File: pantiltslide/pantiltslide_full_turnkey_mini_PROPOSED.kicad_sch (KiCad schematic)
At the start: 64 parts, among them J1 Conn_01x22_Socket, J17 Motor_Slide, J18 Motor_Pan, J19 Motor_Tilt, J2 Conn_01x22_Socket, J20 TCA9548A_Mux, J21 AS5600_Pan, J22 AS5600_Tilt, J23 OLED, J24 TCA9548A_Mux, J26 Limit_Min, J27 Limit_Max, J28 Motor_Aux, J29 Enc_Slide, J3 MUX_2, J30 Enc_Pan, J31 Enc_Tilt, J32 Enc_Aux, J33 Btn_SetKeyframe, J34 Btn_ClearKeyframe, J35 Btn_PlayPause, J36 Btn_Reset, J37 5V_In, J38 24V_In, J4 MUX_3, J41 Aux_Max, J5 MUX_4, J6 MUX_5, J7 MUX_6, J8 MUX_7, U1 tmc2209, U2 tmc2209, U3 tmc2209, U4 tmc2209

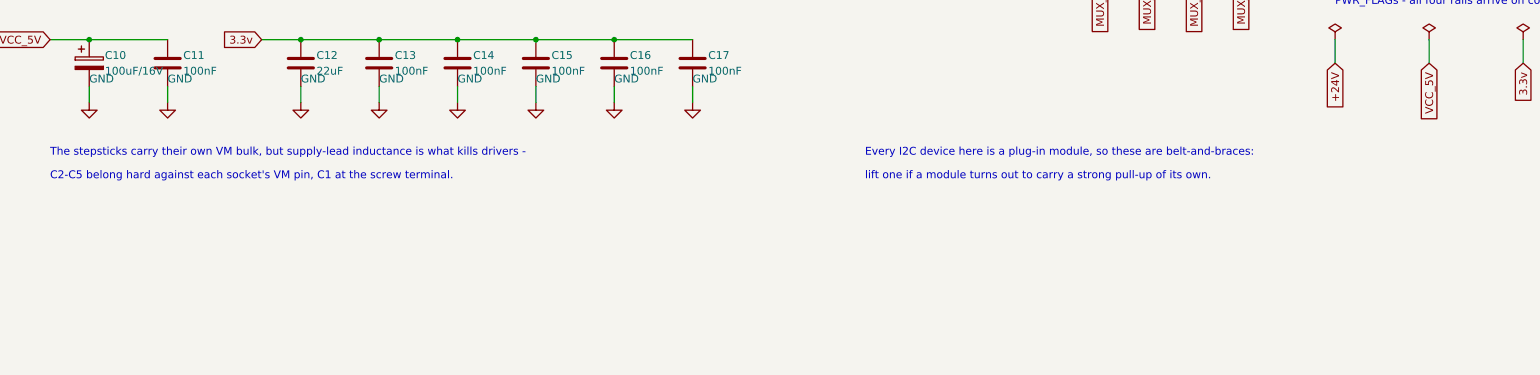
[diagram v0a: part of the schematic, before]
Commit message: new version of board with more caps and res
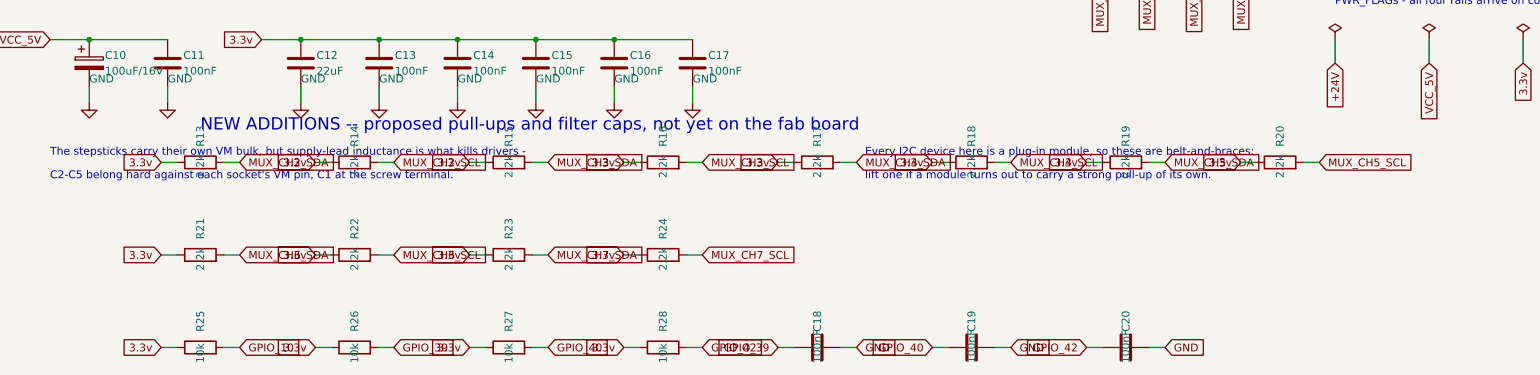
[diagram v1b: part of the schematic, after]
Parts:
- added C18, C19, C20: 100nF, Capacitor_SMD:C_0805_2012Metric, symbol Device:C
- added R13, R14, R15, R16, R17, R18, R19, R20, R21, R22, R23, R24: 2.2k, Resistor_SMD:R_0805_2012Metric, symbol Device:R
- added R25, R26, R27, R28: 10k, Resistor_SMD:R_0805_2012Metric, symbol Device:R
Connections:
- net +3.3V: now also R13.1, R14.1, R15.1, R16.1, R17.1, R18.1, R19.1, R20.1, R21.1, R22.1, R23.1, R24.1, R25.1, R26.1, R27.1, R28.1
- net GND: now also C18.2, C19.2, C20.2
- net GPIO_10: now also R25.2
- net GPIO_39: now also C18.1, R26.2
- net GPIO_40: now also C19.1, R27.2
- net GPIO_42: now also C20.1, R28.2
- net MUX_CH2_SCL: now also R14.2
- net MUX_CH2_SDA: now also R13.2
- net MUX_CH3_SCL: now also R16.2
- net MUX_CH3_SDA: now also R15.2
- net MUX_CH4_SCL: now also R18.2
- net MUX_CH4_SDA: now also R17.2
- net MUX_CH5_SCL: now also R20.2
- net MUX_CH5_SDA: now also R19.2
- net MUX_CH6_SCL: now also R22.2
- net MUX_CH6_SDA: now also R21.2
- net MUX_CH7_SCL: now also R24.2
- net MUX_CH7_SDA: now also R23.2
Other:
- note added: "NEW ADDITIONS -- proposed pull-ups and filter caps, not yet on the fab board"
